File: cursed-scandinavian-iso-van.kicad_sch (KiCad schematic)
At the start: 105 parts, among them J1 Conn_01x04, SW1 SW_Push, U1 ATmega32U4-A, Y1 16MHz

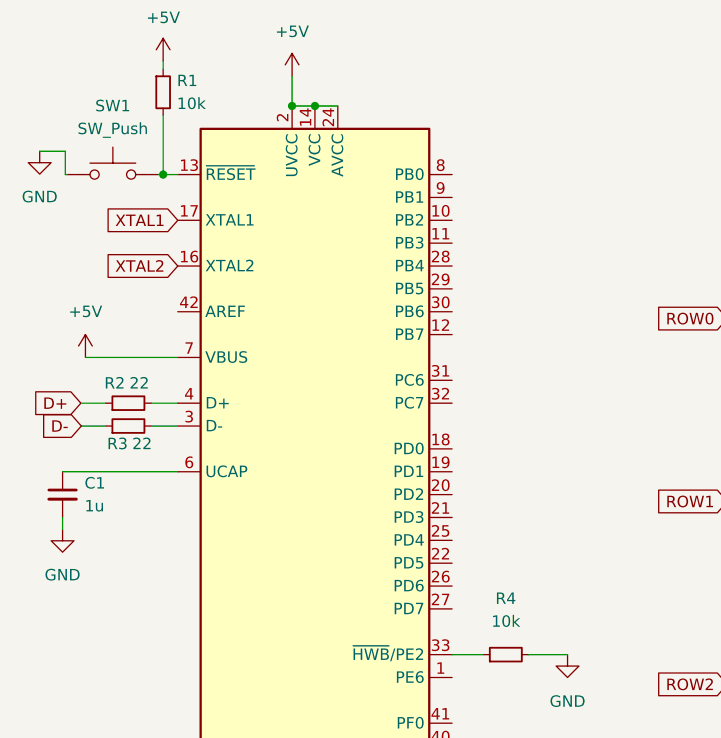
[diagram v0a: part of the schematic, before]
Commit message: maybe all the columns
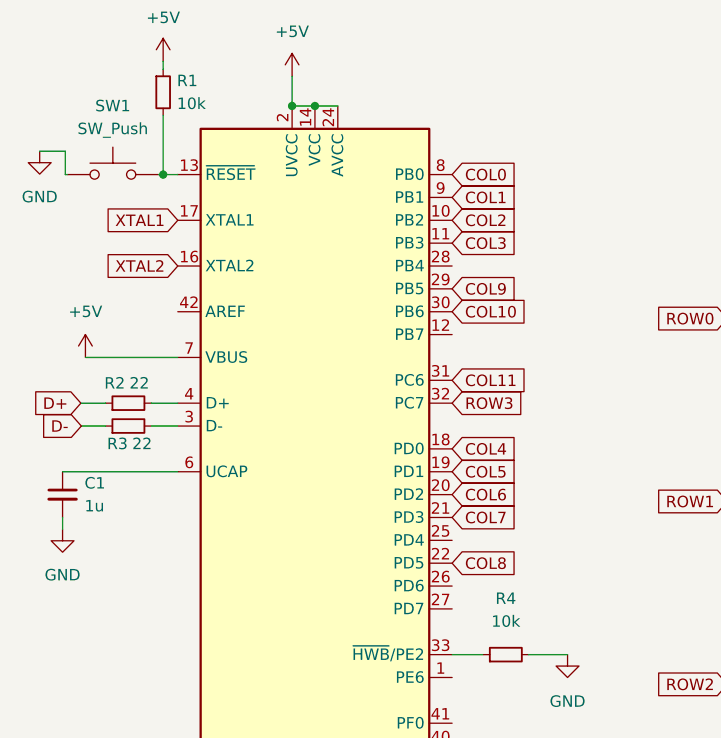
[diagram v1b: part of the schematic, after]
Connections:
- net COL0: now also U1.8 (PB0)
- net COL1: now also U1.9 (PB1)
- net COL10: now also U1.30 (PB6)
- net COL11: now also U1.31 (PC6)
- net COL2: now also U1.10 (PB2)
- net COL3: now also U1.11 (PB3)
- net COL4: now also U1.18 (PD0)
- net COL5: now also U1.19 (PD1)
- net COL6: now also U1.20 (PD2)
- net COL7: now also U1.21 (PD3)
- net COL8: now also U1.22 (PD5)
- net COL9: now also U1.29 (PB5)
- net GND: now also SW1.2; no longer SW1.1
- net ROW3: now also U1.32 (PC7)
- net at R1.2, U1.13 (~{RESET}): now also SW1.1; no longer SW1.2
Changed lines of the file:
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@@
+    )
+  )
+  (global_label "COL9" (shape input) (at 61.4172 45.3136 0) (fields_autoplaced)
+    (effects (font (size 1.27 1.27)) (justify left))
+    (property "Intersheetrefs" "${INTERSHEET_REFS}" (at 69.2405 45.3136 0)
+      (effects (font (size 1.27 1.27)) (justify left) hide)
     )
   )
@@
     )
   )
+  (global_label "COL8" (shape input) (at 61.4172 75.7936 0) (fields_autoplaced)
+    (effects (font (size 1.27 1.27)) (justify left))
+    (property "Intersheetrefs" "${INTERSHEET_REFS}" (at 69.2405 75.7936 0)
+      (effects (font (size 1.27 1.27)) (justify left) hide)
+    )
+  )
   (global_label "COL9" (shape input) (at 234.2896 28.2448 90) (fields_autoplaced)
     (effects (font (size 1.27 1.27)) (justify left))
@@
     )
   )
+  (global_label "COL10" (shape input) (at 61.4172 47.8536 0) (fields_autoplaced)
+    (effects (font (size 1.27 1.27)) (justify left))
+    (property "Intersheetrefs" "${INTERSHEET_REFS}" (at 70.45 47.8536 0)
+      (effects (font (size 1.27 1.27)) (justify left) hide)
+    )
+  )
+  (global_label "COL0" (shape input) (at 61.4172 32.6136 0) (fields_autoplaced)
+    (effects (font (size 1.27 1.27)) (justify left))
+    (property "Intersheetrefs" "${INTERSHEET_REFS}" (at 69.2405 32.6136 0)
+      (effects (font (size 1.27 1.27)) (justify left) hide)
+    )
+  )
+  (global_label "COL3" (shape input) (at 61.4172 40.2336 0) (fields_autoplaced)
+    (effects (font (size 1.27 1.27)) (justify left))
+    (property "Intersheetrefs" "${INTERSHEET_REFS}" (at 69.2405 40.2336 0)
+      (effects (font (size 1.27 1.27)) (justify left) hide)
+    )
+  )
   (global_label "COL5" (shape input) (at 173.3296 28.2448 90) (fields_autoplaced)
     (effects (font (size 1.27 1.27)) (justify left))
     (property "Intersheetrefs" "${INTERSHEET_REFS}" (at 173.3296 20.4215 90)
+      (effects (font (size 1.27 1.27)) (justify left) hide)
+    )
+  )
+  (global_label "COL11" (shape input) (at 61.4172 55.4736 0) (fields_autoplaced)
+    (effects (font (size 1.27 1.27)) (justify left))
+    (property "Intersheetrefs" "${INTERSHEET_REFS}" (at 70.45 55.4736 0)
       (effects (font (size 1.27 1.27)) (justify left) hide)
     )
@@
     )
   )
+  (global_label "COL6" (shape input) (at 61.4172 68.1736 0) (fields_autoplaced)
+    (effects (font (size 1.27 1.27)) (justify left))
+    (property "Intersheetrefs" "${INTERSHEET_REFS}" (at 69.2405 68.1736 0)
+      (effects (font (size 1.27 1.27)) (justify left) hide)
+    )
+  )
   (global_label "XTAL2" (shape input) (at 30.9372 42.7736 180) (fields_autoplaced)
     (effects (font (size 1.27 1.27)) (justify right))
@@
     )
   )
+  (global_label "COL4" (shape input) (at 61.4172 63.0936 0) (fields_autoplaced)
+    (effects (font (size 1.27 1.27)) (justify left))
+    (property "Intersheetrefs" "${INTERSHEET_REFS}" (at 69.2405 63.0936 0)
+      (effects (font (size 1.27 1.27)) (justify left) hide)
+    )
+  )
+  (global_label "COL2" (shape input) (at 61.4172 37.6936 0) (fields_autoplaced)
+    (effects (font (size 1.27 1.27)) (justify left))
+    (property "Intersheetrefs" "${INTERSHEET_REFS}" (at 69.2405 37.6936 0)
+      (effects (font (size 1.27 1.27)) (justify left) hide)
+    )
+  )
   (global_label "COL1" (shape input) (at 112.3696 28.2448 90) (fields_autoplaced)
     (effects (font (size 1.27 1.27)) (justify left))
     (property "Intersheetrefs" "${INTERSHEET_REFS}" (at 112.3696 20.4215 90)
+      (effects (font (size 1.27 1.27)) (justify left) hide)
+    )
+  )
+  (global_label "COL5" (shape input) (at 61.4172 65.6336 0) (fields_autoplaced)
+    (effects (font (size 1.27 1.27)) (justify left))
+    (property "Intersheetrefs" "${INTERSHEET_REFS}" (at 69.2405 65.6336 0)
       (effects (font (size 1.27 1.27)) (justify left) hide)
     )
@@
     (property "Intersheetrefs" "${INTERSHEET_REFS}" (at 83.7522 48.6156 0)
       (effects (font (size 1.27 1.27)) (justify right) hide)
+    )
+  )
+  (global_label "ROW3" (shape input) (at 61.4172 58.0136 0) (fields_autoplaced)
+    (effects (font (size 1.27 1.27)) (justify left))
+    (property "Intersheetrefs" "${INTERSHEET_REFS}" (at 69.6638 58.0136 0)
+      (effects (font (size 1.27 1.27)) (justify left) hide)
+    )
+  )
+  (global_label "COL7" (shape input) (at 61.4172 70.7136 0) (fields_autoplaced)
+    (effects (font (size 1.27 1.27)) (justify left))
+    (property "Intersheetrefs" "${INTERSHEET_REFS}" (at 69.2405 70.7136 0)
+      (effects (font (size 1.27 1.27)) (justify left) hide)
+    )
+  )
+  (global_label "COL1" (shape input) (at 61.4172 35.1536 0) (fields_autoplaced)
+    (effects (font (size 1.27 1.27)) (justify left))
+    (property "Intersheetrefs" "${INTERSHEET_REFS}" (at 69.2405 35.1536 0)
+      (effects (font (size 1.27 1.27)) (justify left) hide)
     )
   )
@@
     )
   )
-  (symbol (lib_id "Switch:SW_Push") (at 23.7236 32.6136 0) (unit 1)
-    (in_bom yes) (on_board yes) (dnp no) (fields_autoplaced)
+  (symbol (lib_id "Switch:SW_Push") (at 23.7236 32.6136 0) (mirror y) (unit 1)
+    (in_bom yes) (on_board yes) (dnp no)
     (property "Reference" "SW1" (at 23.7236 24.9936 0)
       (effects (font (size 1.27 1.27)))
